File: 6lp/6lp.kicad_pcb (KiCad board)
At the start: 2 copper layers, 25.4 x 27.9 mm, 36 parts, among them J1 MODULE_HEADER, T1 2450BM15A0015, U1 AT86RF233, X1 16.0000MF09Z-AC3

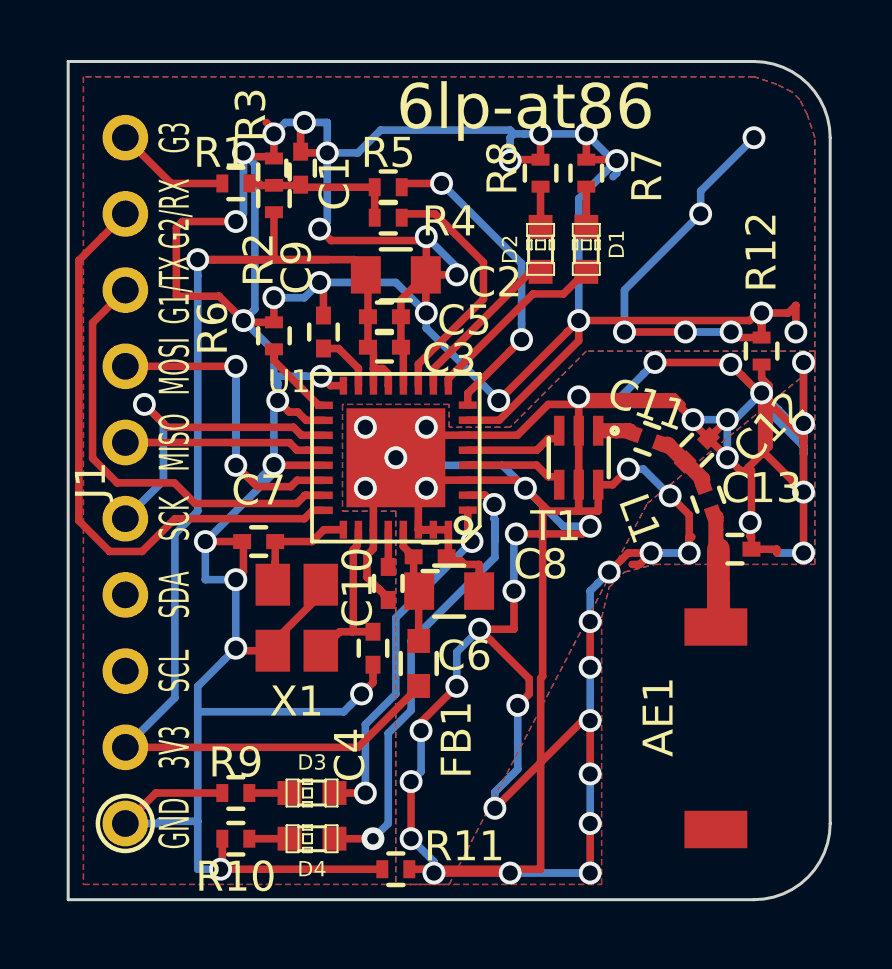
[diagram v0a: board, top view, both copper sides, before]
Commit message: damn you, apc
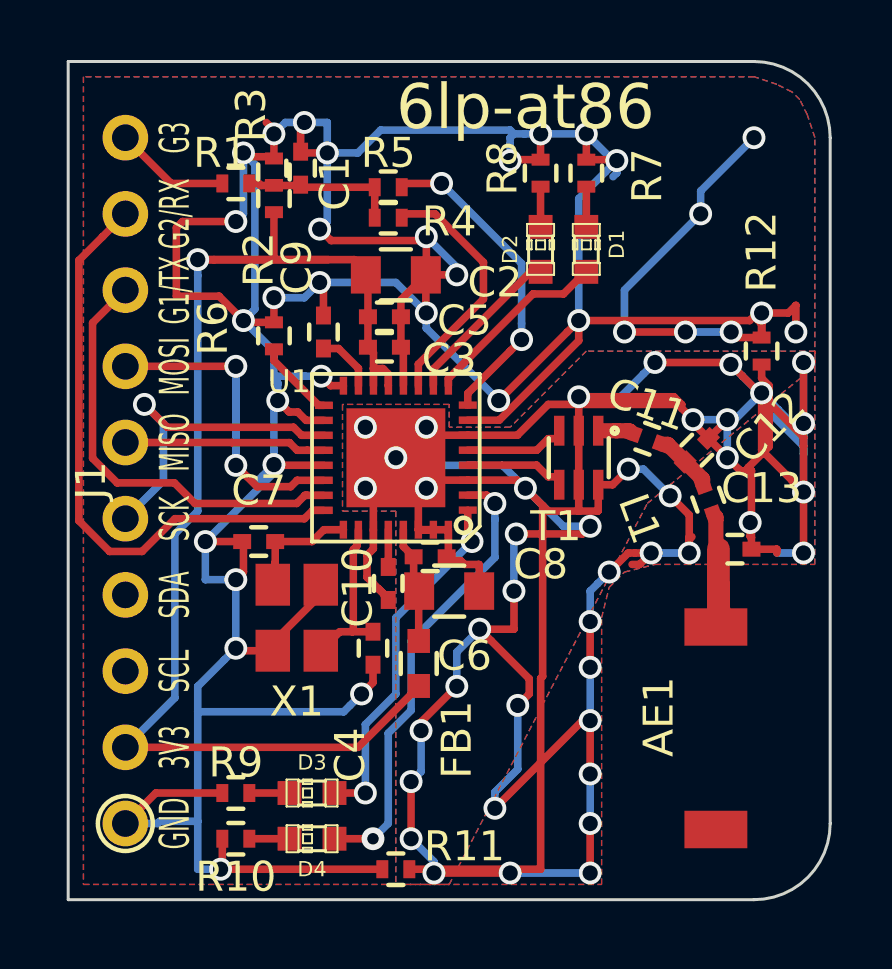
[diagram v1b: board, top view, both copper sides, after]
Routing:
- net /DIG4: track 15.8 -> 15.2 mm
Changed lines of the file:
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@@
     (thickness 1.6)
     (drawings 7)
-    (tracks 602)
+    (tracks 600)
     (zones 0)
     (modules 36)
@@
   )
   (setup
-    (last_trace_width 0.508)
+    (last_trace_width 0.254)
     (trace_clearance 0.2032)
     (zone_clearance 0.2286)
@@
     (visible_elements FFFFFF7F)
     (pcbplotparams
-      (layerselection 0x010b8_80000001)
+      (layerselection 0x010f8_80000001)
       (usegerberextensions false)
       (excludeedgelayer true)
@@
   (segment (start 136.906 123.444) (end 136.906 121.158) (width 0.254) (layer B.Cu) (net 17))
   (segment (start 134.3787 123.444) (end 133.038 123.444) (width 0.254) (layer F.Cu) (net 18) (status 20))
+  (segment (start 140.31976 113.51514) (end 140.94714 113.51514) (width 0.254) (layer F.Cu) (net 19))
+  (segment (start 140.94714 113.51514) (end 141.224 113.792) (width 0.254) (layer F.Cu) (net 19))
+  (segment (start 141.224 114.330815) (end 141.224 113.792) (width 0.254) (layer B.Cu) (net 19))
   (via (at 137.16 124.968) (size 0.762) (layers F.Cu B.Cu) (net 19))
   (segment (start 137.16 124.968) (end 135.8773 124.968) (width 0.254) (layer F.Cu) (net 19))
-  (segment (start 141.224 115.023447) (end 141.224 114.330815) (width 0.254) (layer B.Cu) (net 19))
   (segment (start 141.224 115.591646) (end 141.224 114.330815) (width 0.254) (layer B.Cu) (net 19))
   (segment (start 138.43 118.385646) (end 141.224 115.591646) (width 0.254) (layer B.Cu) (net 19))
@@
   (segment (start 137.668 124.46) (end 137.668 121.451426) (width 0.254) (layer B.Cu) (net 19))
   (segment (start 137.16 124.968) (end 137.668 124.46) (width 0.254) (layer B.Cu) (net 19))
-  (segment (start 140.31976 113.51514) (end 140.890951 113.51514) (width 0.254) (layer F.Cu) (net 19))
-  (segment (start 141.199833 114.306648) (end 141.199833 113.824022) (width 0.254) (layer B.Cu) (net 19))
-  (via (at 141.199833 113.824022) (size 0.762) (drill 0.508) (layers F.Cu B.Cu) (net 19))
-  (segment (start 140.890951 113.51514) (end 141.199833 113.824022) (width 0.254) (layer F.Cu) (net 19))
-  (segment (start 141.224 114.330815) (end 141.199833 114.306648) (width 0.254) (layer B.Cu) (net 19))
+  (via (at 141.224 113.792) (size 0.762) (drill 0.508) (layers F.Cu B.Cu) (net 19))
   (segment (start 134.3787 124.968) (end 133.038 124.968) (width 0.254) (layer F.Cu) (net 20) (status 20))
   (via (at 129.54 110.49) (size 0.762) (drill 0.508) (layers F.Cu B.Cu) (net 23))
